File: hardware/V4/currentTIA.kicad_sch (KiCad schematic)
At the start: 24 parts, among them Q10 MMBFJ112, Q3 MMBFJ112, Q4 MMBFJ112, Q5 BCM856BSH-Q, Q6 MMBFJ112, Q7 MMBFJ112, Q8 MMBFJ112, Q9 2PD601ARL

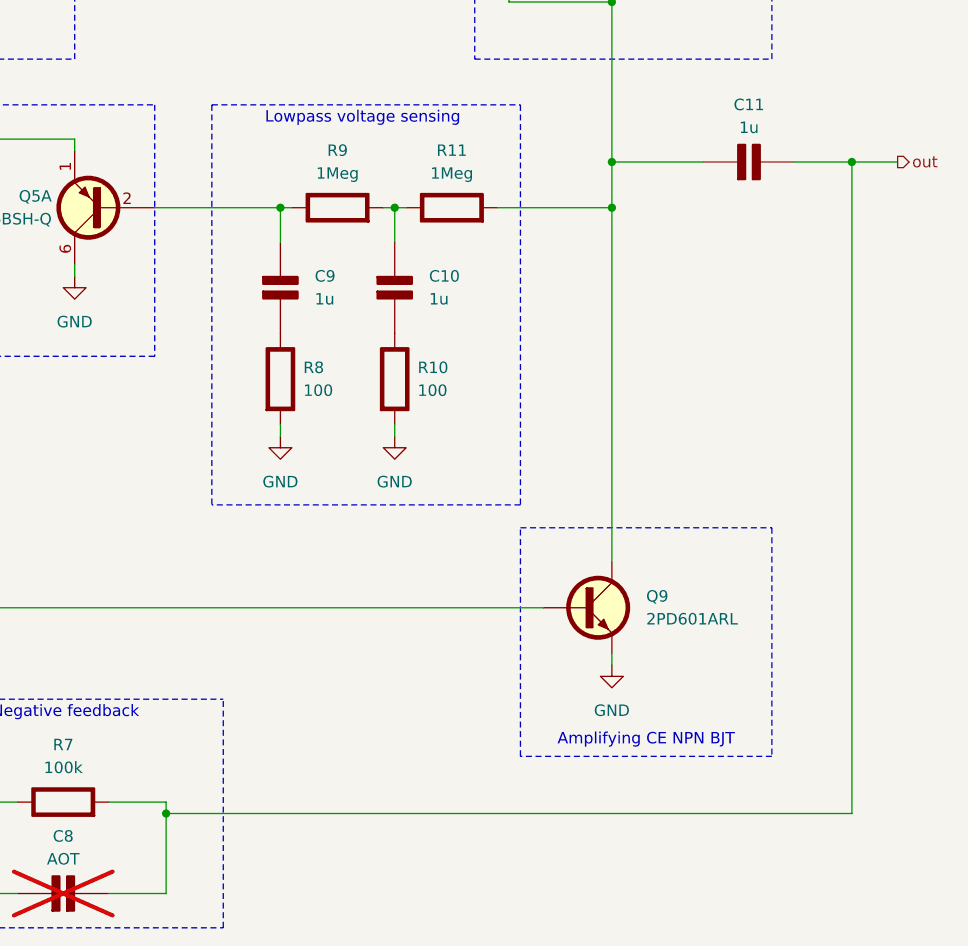
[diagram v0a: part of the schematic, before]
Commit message: Adding initial v4 design
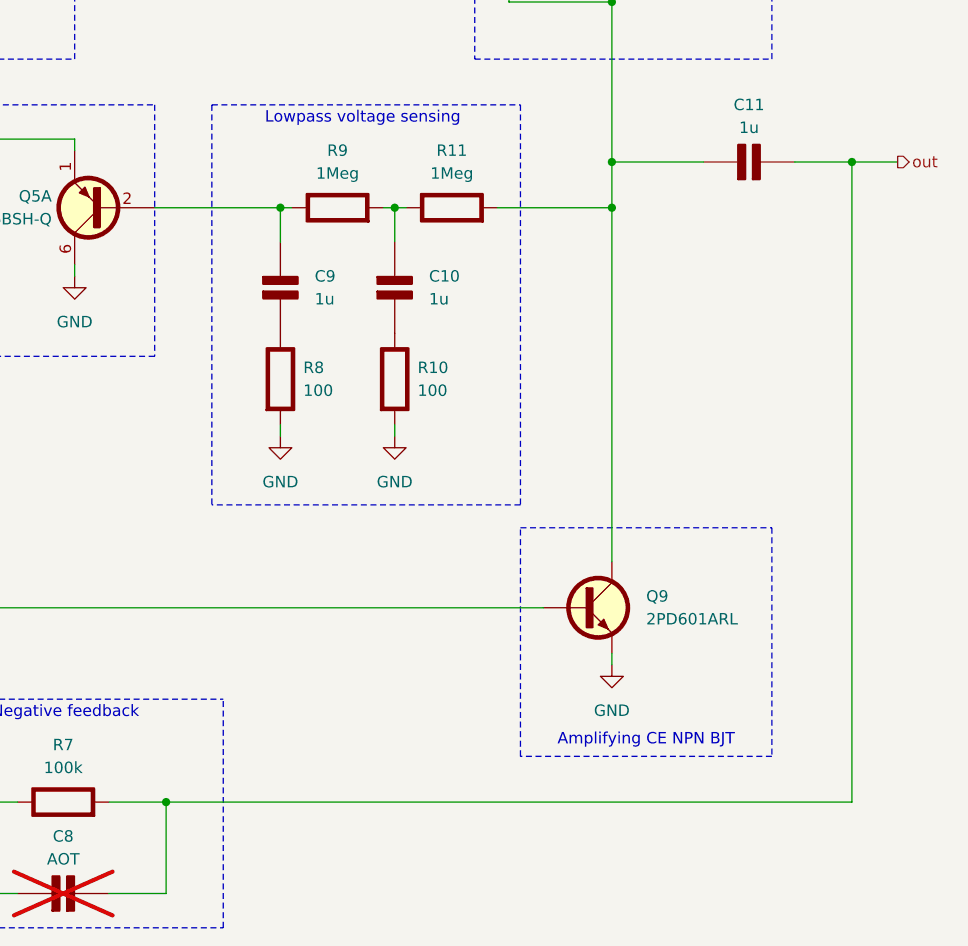
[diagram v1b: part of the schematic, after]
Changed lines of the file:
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@@
+	)
+	(junction
+		(at 158.75 158.75)
+		(diameter 0)
+		(color 0 0 0 0)
 	)
 	(junction
@@
 	)
 	(junction
-		(at 158.75 160.02)
-		(diameter 0)
-		(color 0 0 0 0)
-	)
-	(junction
 		(at 73.66 71.12)
 		(diameter 0)
@@
 	(wire
 		(pts
-			(xy 158.75 160.02) (xy 158.75 158.75)
+			(xy 158.75 158.75) (xy 158.75 168.91)
 		)
 		(stroke
@@
 	(wire
 		(pts
-			(xy 234.95 87.63) (xy 234.95 160.02)
+			(xy 234.95 87.63) (xy 234.95 158.75)
 		)
 		(stroke
@@
 	(wire
 		(pts
-			(xy 158.75 160.02) (xy 234.95 160.02)
+			(xy 158.75 158.75) (xy 234.95 158.75)
 		)
 		(stroke
@@
 		)
 		(stroke
-			(width 0)
-			(type default)
-		)
-	)
-	(wire
-		(pts
-			(xy 158.75 168.91) (xy 158.75 160.02)
-		)
-		(stroke
